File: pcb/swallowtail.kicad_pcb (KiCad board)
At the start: 2 copper layers, 134.5 x 111.9 mm, 114 parts, among them J1 MJ-4PP-9, J2 Conn_01x04, SW1 SW_PUSH, SW10 SW_PUSH, SW11 SW_PUSH, SW12 SW_PUSH, SW13 SW_PUSH, SW14 SW_PUSH, SW15 SW_PUSH, SW16 SW_PUSH, SW17 SW_PUSH, SW18 SW_PUSH, SW19 SW_PUSH, SW2 SW_PUSH, SW20 SW_PUSH, SW21 SW_PUSH, SW22 SW_PUSH, SW23 SW_PUSH, SW24 SW_PUSH, SW25 SW_PUSH, SW26 SW_PUSH, SW27 SW_PUSH, SW28 SW_PUSH, SW29 SW_PUSH, SW3 SW_PUSH, SW30 SW_PUSH, SW4 SW_PUSH, SW5 SW_PUSH, SW6 SW_PUSH, SW7 SW_PUSH, SW8 SW_PUSH, SW9 SW_PUSH, U1 ProMicro_r

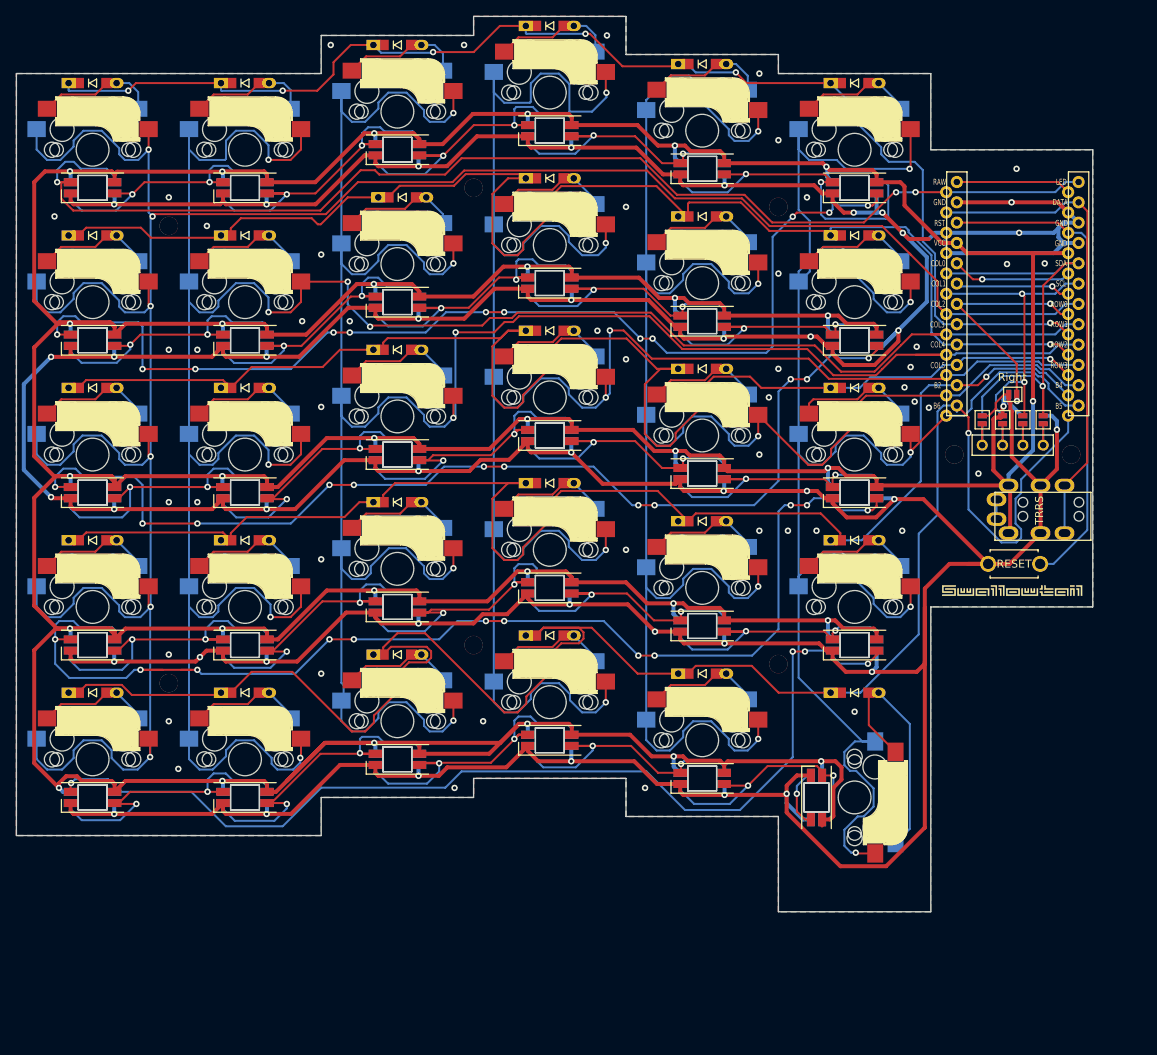
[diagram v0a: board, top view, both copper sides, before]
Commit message: v2 design
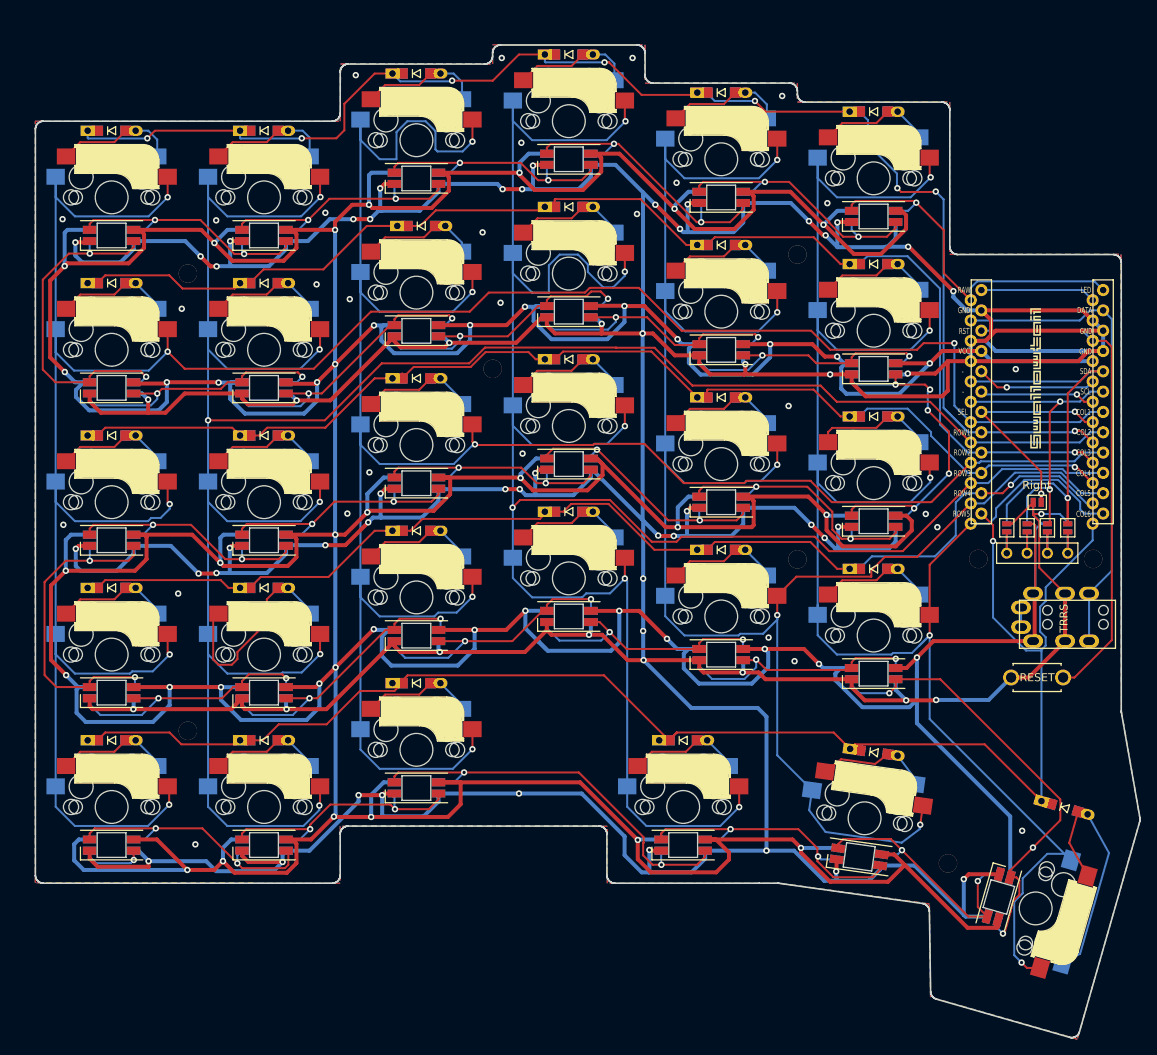
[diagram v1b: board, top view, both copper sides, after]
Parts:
- removed the G*** at (159.0, 115.8) (x2)
- removed the Ref** at (166.4, 98.8)
- removed the Ref** at (151.8, 98.8)
- removed the Ref** at (129.8, 67.9)
- removed the Ref** at (129.8, 125.0)
- removed the Ref** at (91.7, 65.5)
- removed the Ref** at (91.7, 122.6)
- removed the Ref** at (53.6, 127.4)
- removed the Ref** at (53.6, 70.2)
- added G***: LOGO, swallowtail:tiny_logo, B.Cu at (161.9, 89.3)
- added G***: LOGO, swallowtail:tiny_logo, F.Cu at (161.9, 89.3)
- added Ref**: Val**, kbd:M2_Threads_v2, F.Cu at (169.1, 111.9)
- added Ref**: Val**, kbd:M2_Threads_v2, F.Cu at (154.8, 111.9)
- added Ref**: Val**, kbd:M2_Threads_v2, F.Cu at (132.2, 111.9)
- added Ref**: Val**, kbd:M2_Threads_v2, F.Cu at (132.2, 73.8)
- added Ref**: Val**, kbd:M2_Threads_v2, F.Cu at (94.1, 88.1)
- added Ref**: Val**, kbd:M2_Threads_v2, F.Cu at (151.0, 149.9)
- added Ref**: Val**, kbd:M2_Threads_v2, F.Cu at (56.0, 133.4)
- added Ref**: Val**, kbd:M2_Threads_v2, F.Cu at (56.0, 76.2)
- LED1, LED10, LED11, LED12, LED13, LED14, LED15, LED16, LED17, LED18, LED19, LED2, LED20, LED21, LED22, LED23, LED24, LED25, LED26, LED27, LED28, LED29, LED3, LED30, LED4, LED5, LED6, LED7, LED8, LED9: footprint kbd:YS-SK6812MINI-E_reversible -> swallowtail:YS-SK6812MINI-E_reversible_no_edge_cuts
- U1: footprint kbd:ProMicro_v2 -> swallowtail:ProMicro_v2_mod
- moved LED25 114.0 mm to (157.3, 154.1), turned to 254 degrees
- moved LED13 97.7 mm to (141.7, 107.2)
- moved LED1 97.7 mm to (141.7, 69.1)
- moved LED18 93.1 mm to (46.4, 109.5)
- moved LED6 93.1 mm to (46.4, 71.4)
- moved LED30 88.3 mm to (46.4, 147.6), turned to 0 degrees
- moved LED26 77.1 mm to (139.9, 149.1), turned to 352 degrees
- moved LED14 59.5 mm to (122.6, 104.8)
- moved LED2 59.5 mm to (122.6, 66.7)
- moved LED29 55.4 mm to (65.5, 147.6)
- moved LED17 55.4 mm to (65.5, 109.5)
- moved LED5 55.4 mm to (65.5, 71.4)
- moved LED27 37.3 mm to (117.9, 147.6)
- moved D30 29.9 mm to (165.5, 143.0), turned to 344 degrees
- moved SW30 26.5 mm to (161.9, 155.6), turned to 254 degrees
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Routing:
- net VCC: track 888.2 -> 1142.5 mm, vias 32 -> 46
- net GND: track 874.0 -> 982.4 mm, vias 92 -> 96
- net Net-(LED18-Pad2): track 147.7 -> 41.4 mm, vias 12 -> 2
- net D3: track 151.8 -> 46.0 mm, vias 3 -> 1
- net Net-(LED6-Pad2): track 139.6 -> 43.4 mm, vias 12 -> 2
- net Net-(LED12-Pad2): track 136.6 -> 41.8 mm, vias 12 -> 5
- net Net-(LED24-Pad2): track 127.8 -> 57.6 mm, vias 4 -> 3
- net B6: track 243.1 -> 205.2 mm
- net B3: track 186.4 -> 150.0 mm
- net B2: track 181.7 -> 155.1 mm
- net F7: track 167.8 -> 191.9 mm, vias 6 -> 8
- net D7: track 295.3 -> 273.3 mm, vias 6 -> 5
- net Net-(D20-Pad2): track 14.4 -> 27.4 mm
- net B1: track 177.6 -> 164.9 mm
- net B4: track 248.0 -> 235.7 mm
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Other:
- board size 134.5 x 111.9 mm -> 138.1 x 124.1 mm
